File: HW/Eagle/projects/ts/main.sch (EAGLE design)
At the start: 33 parts, among them IC1 4050D, U1 ATMEGA328P-PU, U2 LM2576T, U3 HT7533, U4 LM75

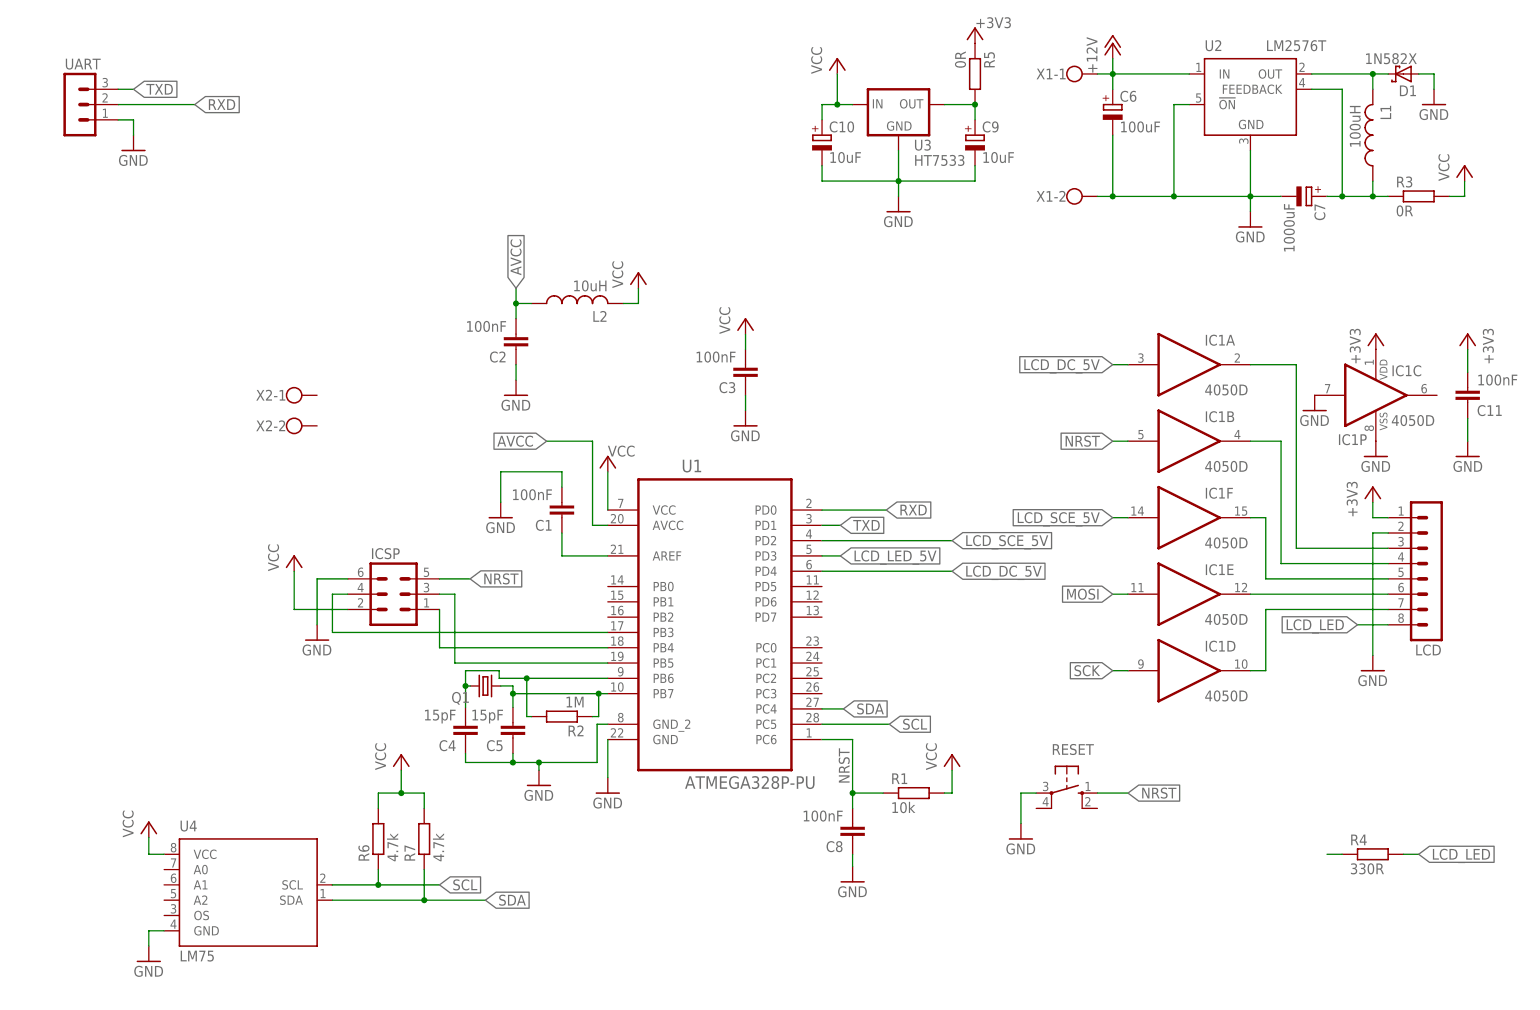
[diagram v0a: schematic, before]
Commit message: Big Update
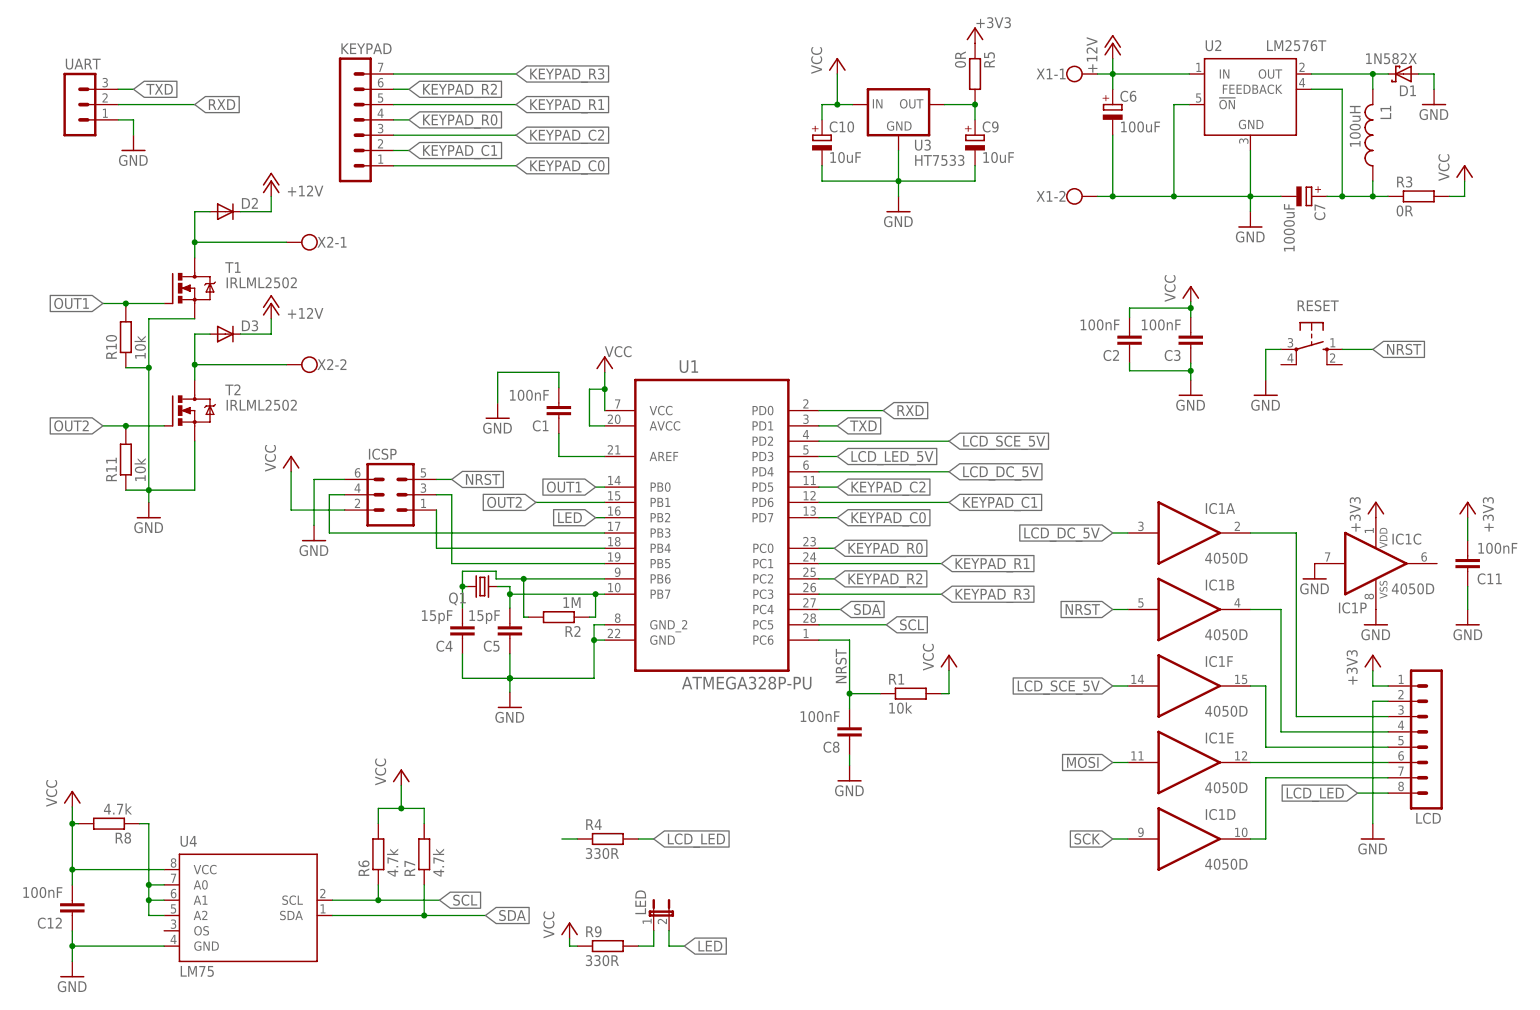
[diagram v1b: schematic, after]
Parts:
- removed L2: 10uH, misc:FERRCORE
- added C12: 100nF, rcl:C-EUC0805
- added D2, D3: (no value), diode:DIODE-MINIMELF
- added KEYPAD: (no value), con-lstb:MA07-1
- added LED: (no value), jumper:JP1E
- added R10, R11: 10k, rcl:R-EU_R0805
- added R8: 4.7k, rcl:R-EU_R0805
- added R9: 330R, rcl:R-EU_R0805
- added T1, T2: IRLML2502, misc:IRLML2502
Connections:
- removed net AVCC: C2.2, L2.1, U1.AVCC
- new net KEYPAD_C0: KEYPAD.1, U1.PD7
- new net KEYPAD_C1: KEYPAD.2, U1.PD6
- new net KEYPAD_C2: KEYPAD.3, U1.PD5
- new net KEYPAD_R0: KEYPAD.4, U1.PC0
- new net KEYPAD_R1: KEYPAD.5, U1.PC1
- new net KEYPAD_R2: KEYPAD.6, U1.PC2
- new net KEYPAD_R3: KEYPAD.7, U1.PC3
- new net LED: LED.2, U1.PB2
- new net N$10: D2.A, T1.D, X2-1.KL
- new net N$11: D3.A, T2.D, X2-2.KL
- new net N$5: R8.1, U4.A0, U4.A1, U4.A2
- new net N$6: LED.1, R9.2
- new net OUT1: R10.2, T1.G, U1.PB0
- new net OUT2: R11.2, T2.G, U1.PB1
- net +12V: now also D2.C, D3.C
- net GND: now also C12.1, R10.1, R11.1, T1.S, T2.S
- net VCC: now also C12.2, C2.2, R8.2, R9.1, U1.AVCC; no longer L2.2
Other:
- moved on the sheet: C1, C11, C2, C3, C4, C5, C8, IC1A, IC1B, IC1C, IC1D, IC1E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
